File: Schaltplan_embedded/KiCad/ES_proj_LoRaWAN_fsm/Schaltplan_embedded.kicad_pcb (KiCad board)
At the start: 2 copper layers, 78 parts, among them IC1 TPS22943DCKR, IC2 BGA824N6E6327XTSA1, IC3 TESEO-LIV3F, IC4 L6924D, IC5 SPV1040T, IC6 TLS850B0TBV33ATMA1, IC7 TLS850B0TBV55ATMA1, J1 Conn_02x05_Odd_Even, J2 Conn_01x02, J3 53048-0810, J4 CONSMA002-L-G, J5 CONSMA002-L-G, J6 CON-SOCJ-2155, J7 Conn_01x02, U1 STM32L476RGTx, U2 RFM92W_93W, Y1 Crystal 8Mhz

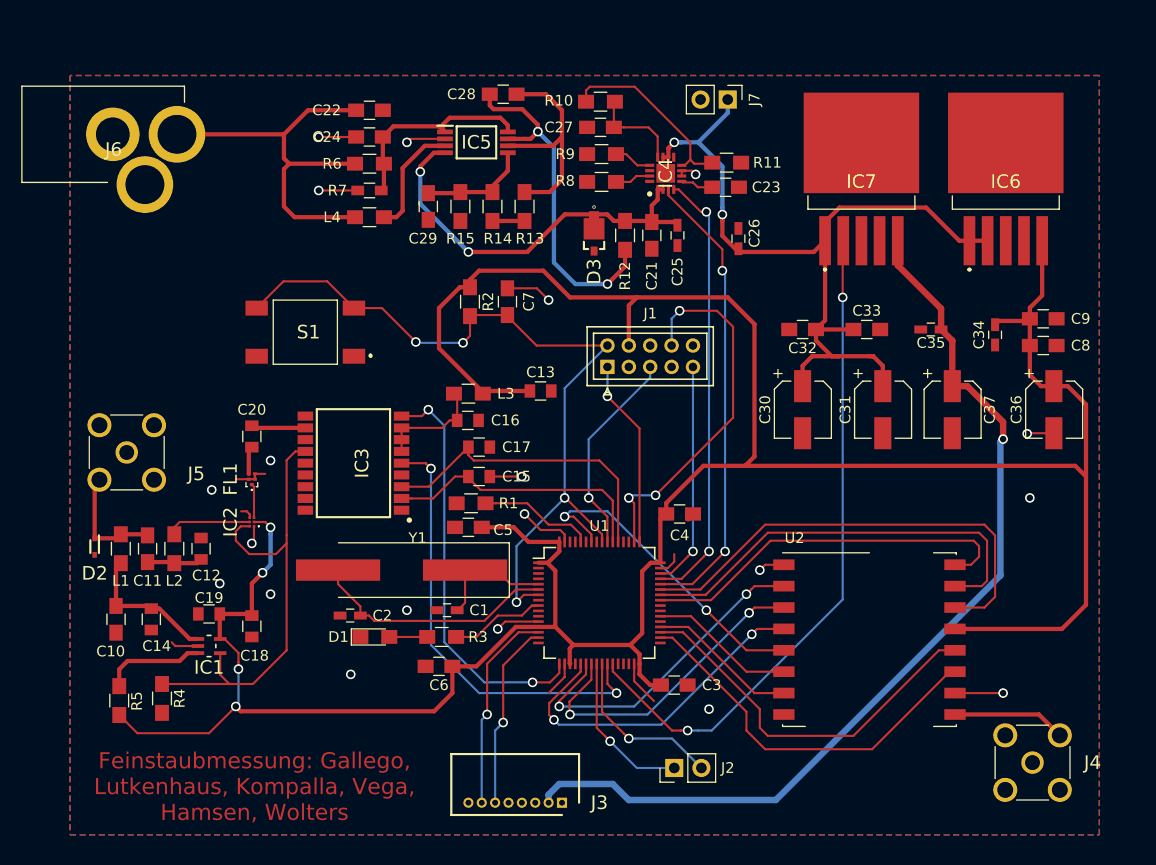
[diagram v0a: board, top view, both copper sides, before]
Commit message: git :)
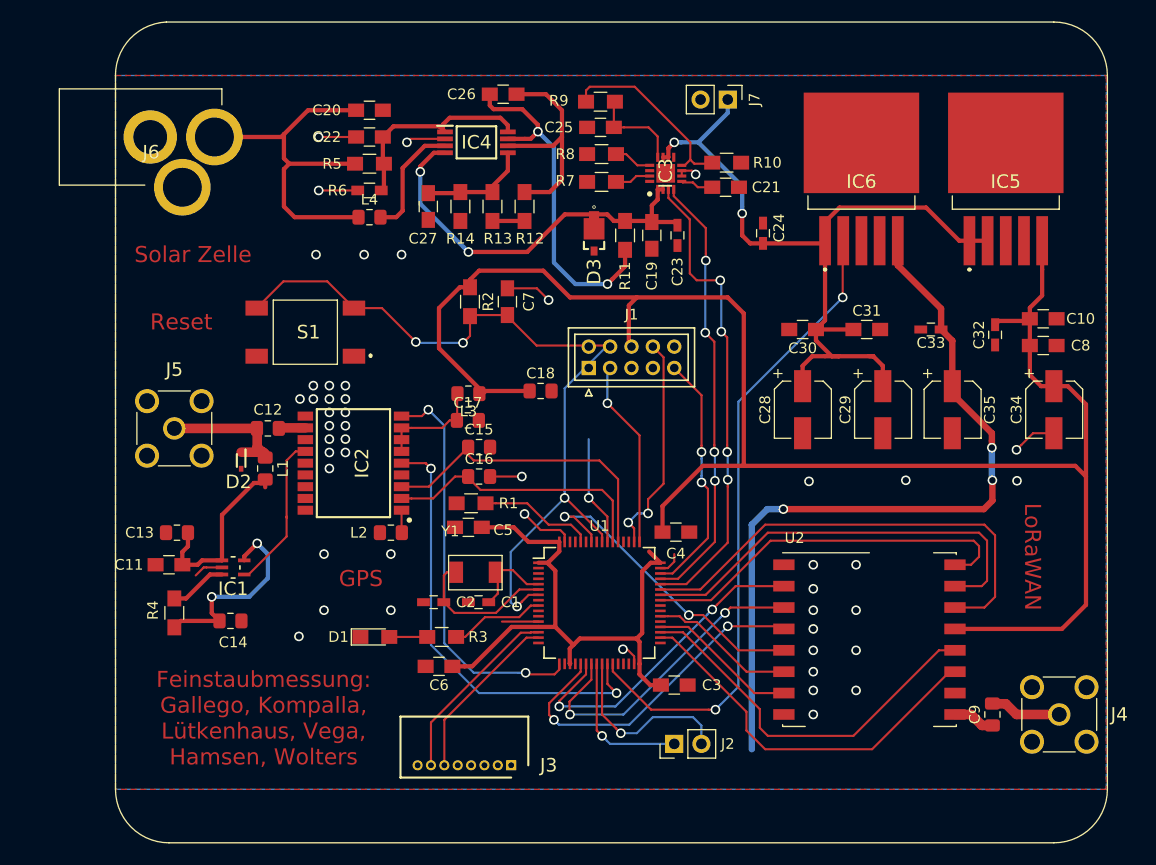
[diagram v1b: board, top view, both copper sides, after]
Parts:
- removed the C11 at (102.2, 89.0)
- removed the C19 at (108.0, 95.1)
- removed the C20 at (112.0, 78.5)
- removed FL1: B4327, SamacSys_Parts:B39162B4353P810
- removed the IC2 at (112.0, 86.5)
- removed the R4 at (103.6, 103.0)
- added C9: 120pF, Capacitor_SMD:C_0805_2012Metric_Pad1.15x1.40mm_HandSolder, F.Cu at (181.2, 104.5)
- C12: value 3.9pF -> 120pF; footprint Capacitors_SMD:C_0805 -> Capacitor_SMD:C_0805_2012Metric_Pad1.15x1.40mm_HandSolder
- C13: value 10nF -> 1uF; footprint Capacitors_SMD:C_0805 -> Capacitor_SMD:C_0805_2012Metric_Pad1.15x1.40mm_HandSolder
- C14: value 1uF -> 2.2uF; footprint Capacitors_SMD:C_0805 -> Capacitor_SMD:C_0805_2012Metric_Pad1.15x1.40mm_HandSolder
- C15, C16, C17: footprint Capacitors_SMD:C_0805 -> Capacitor_SMD:C_0805_2012Metric_Pad1.15x1.40mm_HandSolder
- C18: value 1nF -> 10nF; footprint Capacitors_SMD:C_0805 -> Capacitor_SMD:C_0805_2012Metric_Pad1.15x1.40mm_HandSolder
- L1, L3, L4: footprint Resistors_SMD:R_0805_HandSoldering -> Inductor_SMD:L_0805_2012Metric_Pad1.15x1.40mm_HandSolder
- L2: value 6.8nH -> 100nH; footprint Resistors_SMD:R_0805_HandSoldering -> Inductor_SMD:L_0805_2012Metric_Pad1.15x1.40mm_HandSolder
- Y1: value Crystal 8Mhz -> ECS-80-12-30Q-DS-TR; footprint Crystals:Crystal_SMD_HC49-SD_HandSoldering -> myLib:Quarz
- moved C13 36.5 mm to (105.0, 87.5), turned to 180 degrees
- moved C18 34.8 mm to (139.0, 74.2), turned to 0 degrees
- moved L2 20.3 mm to (125.0, 87.5), turned to 180 degrees
- moved D2 15.9 mm to (111.0, 80.8)
- moved L1 15.4 mm to (113.2, 81.5)
- moved C12 12.9 mm to (113.5, 77.8), turned to 180 degrees
- moved R4 9.68 mm to (104.8, 95.0)
- moved C2 7.90 mm to (129.0, 94.0)
- moved IC1 7.69 mm to (110.2, 90.8)
- moved C14 7.40 mm to (110.0, 95.8), turned to 0 degrees
- moved C11 7.11 mm to (104.2, 90.5), turned to 180 degrees
- moved J3 5.90 mm to (136.2, 109.2)
- moved C16 5.35 mm to (133.2, 82.2)
- moved J4 5.15 mm to (187.5, 104.5)
- moved J5 4.99 mm to (104.8, 77.8)
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- renumbered C9 to C10, C10 to C11, C21 to C19, C22 to C20, C23 to C21, C24 to C22, C25 to C23, C26 to C24, C27 to C25, C28 to C26, C29 to C27, C30 to C28, C31 to C29, C32 to C30, C33 to C31, C34 to C32, C35 to C33, C36 to C34, C37 to C35, IC3 to IC2, IC4 to IC3, IC5 to IC4, IC6 to IC5, IC7 to IC6, R11 to R10, R12 to R11, R13 to R12, R14 to R13, R15 to R14, R5 to R4, R6 to R5, R7 to R6, R8 to R7, R9 to R8, R10 to R9
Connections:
- net AntOFF renamed Net-(IC1-Pad4)
- C11 pad 1: Net-(C10-Pad1) -> Net-(C11-Pad1)
- C12 pad 1: GND -> Net-(C12-Pad1)
- C12 pad 2: Net-(C11-Pad1) -> Net-(C12-Pad2)
- C13 pad 1: +3V3 -> Net-(C11-Pad1)
- C14 pad 1: Net-(C10-Pad1) -> Net-(C14-Pad1)
- C15 pad 1: UART_5_RX -> UART_5_TX
- C16 pad 1: Net-(C16-Pad1) -> UART_5_RX
- C17 pad 1: UART_5_TX -> Net-(C17-Pad1)
- C18 pad 1: GND -> +3V3
- C18 pad 2: +3V3 -> GND
- D2 pad 1: Net-(C11-Pad2) -> Net-(C12-Pad2)
- IC1 pad 1: Net-(C10-Pad1) -> Net-(C11-Pad1)
- IC1 pad 5: +3V3 -> Net-(C14-Pad1)
- IC2 pad 1: GND -> Net-(IC2-Pad1)
- IC2 pad 11: RF_IN -> Net-(C12-Pad1)
- IC2 pad 6: Net-(C16-Pad1) -> Net-(C17-Pad1)
- IC2 pad 7: Net-(C16-Pad1) -> Net-(C17-Pad1)
- IC2 pad 8: Net-(C16-Pad1) -> Net-(C17-Pad1)
- J4 pad 1: GND -> Net-(C9-Pad2)
- J4 pad 5: Net-(J4-Pad5) -> GND
- J5 pad 1: GND -> Net-(C12-Pad2)
- J5 pad 5: Net-(C11-Pad2) -> GND
- L1 pad 1: Net-(C11-Pad2) -> Net-(C12-Pad2)
- L1 pad 2: Net-(C10-Pad1) -> Net-(C11-Pad1)
- L2 pad 1: Net-(C11-Pad1) -> Net-(IC2-Pad1)
- L2 pad 2: Net-(IC2-Pad5) -> GND
- L3 pad 2: Net-(C16-Pad1) -> Net-(C17-Pad1)
- R4 pad 1: +3V3 -> Net-(C14-Pad1)
- U2 pad 9: Net-(J4-Pad5) -> Net-(C9-Pad1)
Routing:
- net +3V3: track 280.7 -> 219.1 mm, vias 4 -> 0
- net Net-(IC1-Pad4): track 44.4 -> 14.7 mm
- net Net-(C14-Pad1): track 0.00 -> 18.8 mm, vias 0 -> 2
- net GND: track 57.7 -> 40.0 mm, vias 20 -> 37
- net +5V: track 89.3 -> 72.6 mm, vias 1 -> 3
- net JTAG_TDI: track 34.9 -> 20.9 mm, vias 3 -> 2
- net Net-(C10-Pad1): track 13.1 -> 0.00 mm
- net Net-(C12-Pad2): track 0.00 -> 12.8 mm
- net Net-(C11-Pad1): track 5.19 -> 17.0 mm
- net Net-(C11-Pad2): track 10.9 -> 0.00 mm
- net Net-(J4-Pad5): track 10.6 -> 0.00 mm
- net Net-(C17-Pad1): track 0.00 -> 10.3 mm
- net Net-(C16-Pad1): track 10.3 -> 0.00 mm
- net Net-(C2-Pad2): track 23.2 -> 13.9 mm
- net JTAG_TDO: track 19.5 -> 10.3 mm
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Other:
- net class Antenna: trace_width 0.4 -> 0.9
- board text added: "Feinstaubmessung: Gallego, Kompalla, Lütkenhaus, Vega, Hamsen, Wolters"
- board text added: "GPS"
- board text added: "LoRaWAN"
- board text added: "Reset"
- board text added: "Solar Zelle"
- board text removed: "Feinstaubmessung: Gallego, Lutkenhaus, Kompalla, Vega, Hamsen, Wolters"
